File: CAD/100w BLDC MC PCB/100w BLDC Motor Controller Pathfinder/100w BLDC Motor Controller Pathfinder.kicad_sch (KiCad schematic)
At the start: 30 parts, among them SW1 PTS815 SJM 250 SMTR LFS, SW2 PTS815 SJM 250 SMTR LFS, U1 RP2040, U2 W25Q128JVS, Y1 ABLS-12.000MHZ-B4-T

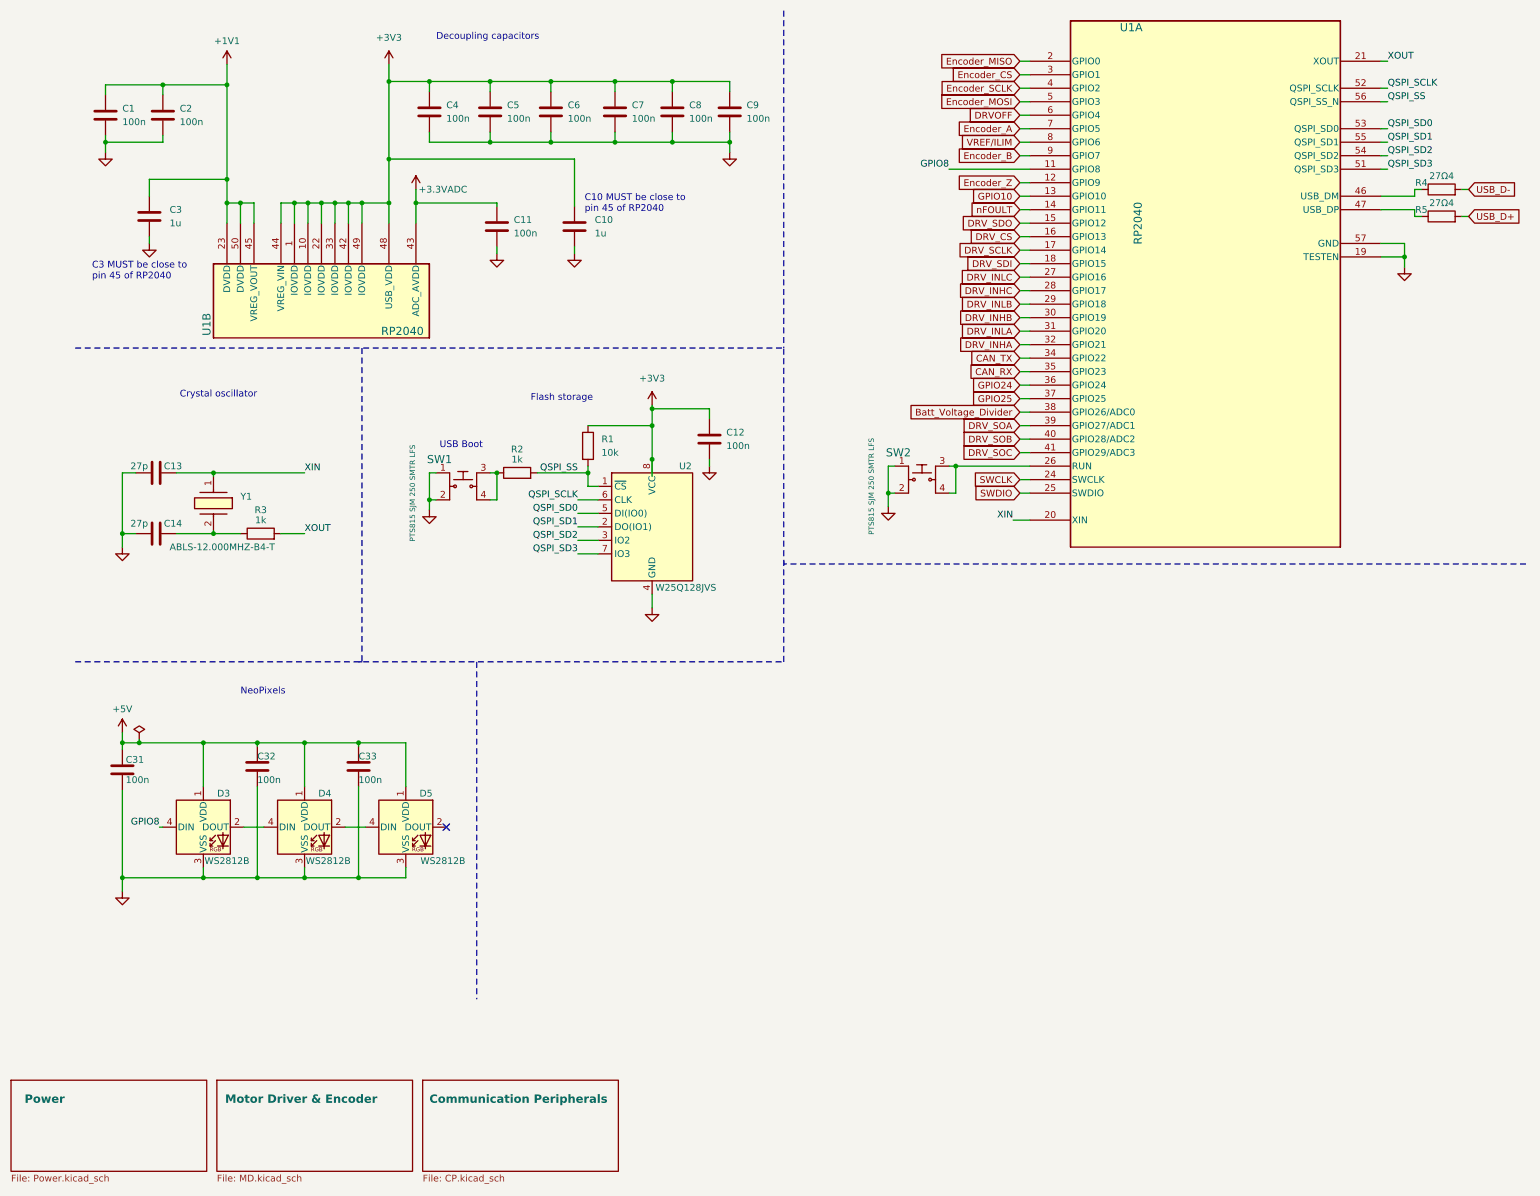
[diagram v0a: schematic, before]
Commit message: Rev: 0.1
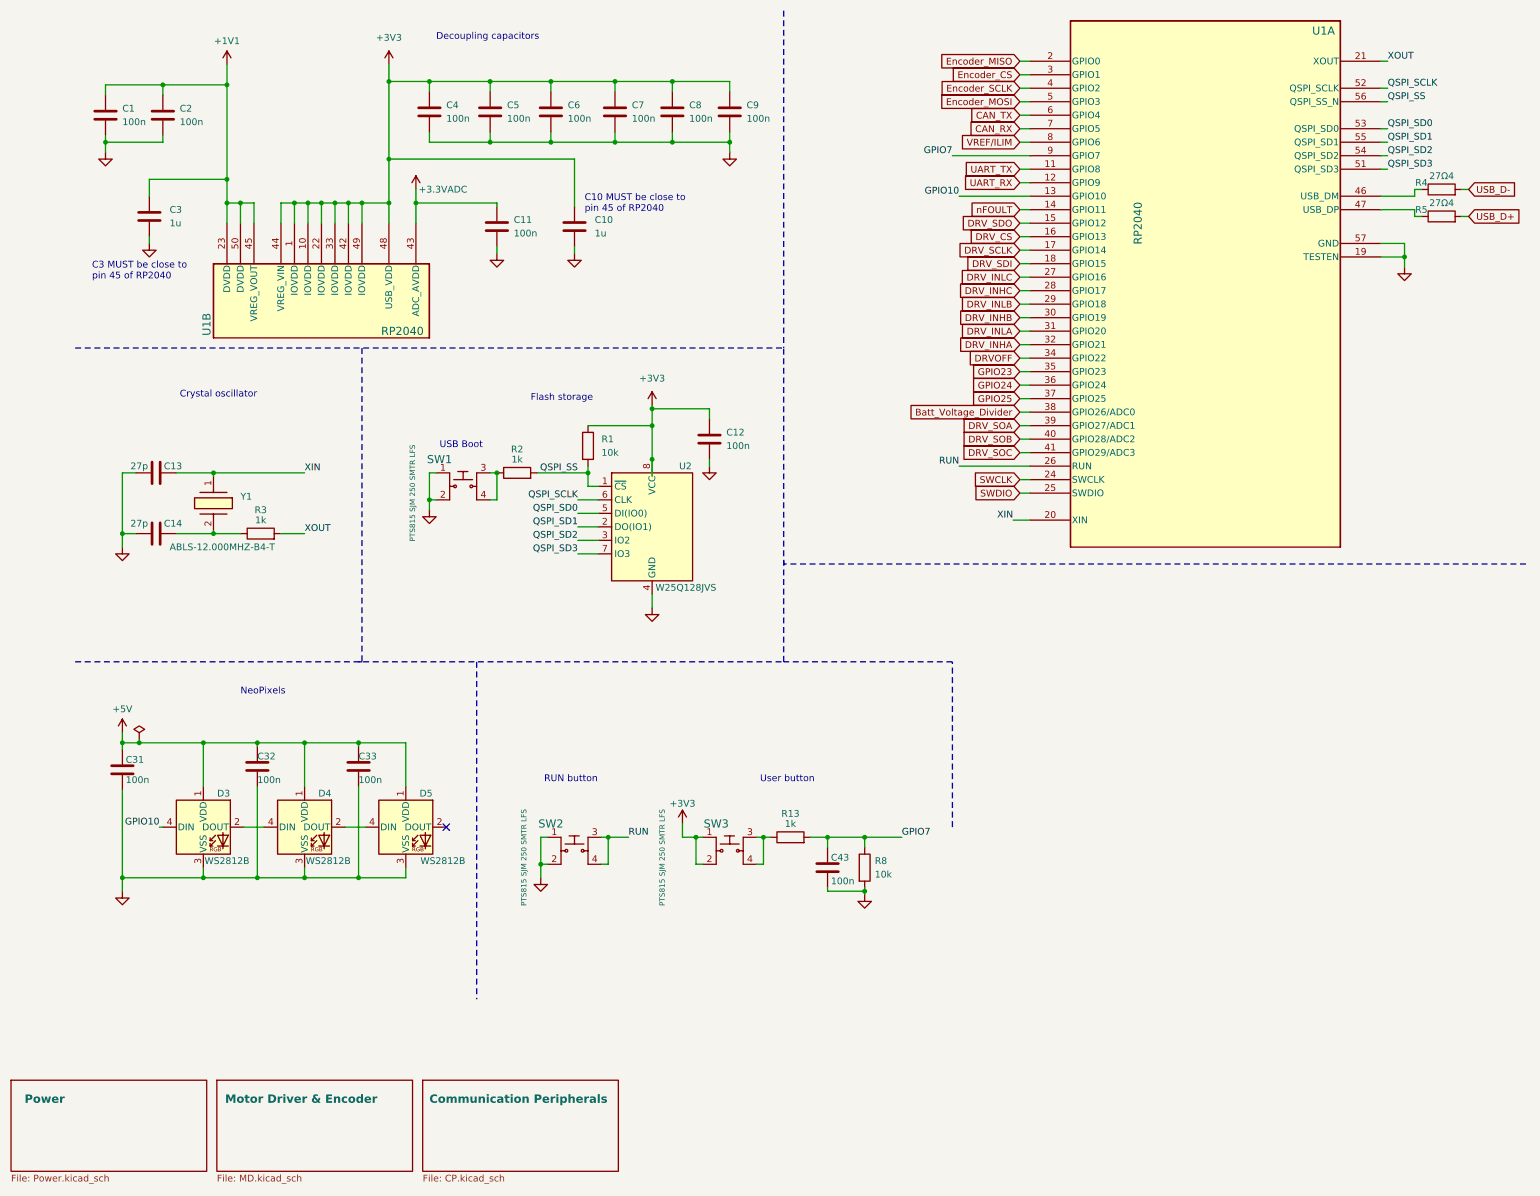
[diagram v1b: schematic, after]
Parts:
- added C43: 100n, symbol Device:C
- added R13: 1k, symbol Device:R
- added R8: 10k, symbol Device:R
- added SW3: PTS815 SJM 250 SMTR LFS, SW4_PTS815 SJM 250 SMTR LFS_CNK, symbol 2024-01-22_02-04-17:PTS815_SJM_250_SMTR_LFS
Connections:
- net Encoder_A is gone; now on net CAN_RX: U1.7 (GPIO5)
- net +3V3: now also SW3.1, SW3.2
- net CAN_RX: no longer U1.35 (GPIO23)
- net CAN_TX: now also U1.6 (GPIO4); no longer U1.34 (GPIO22)
- net DRVOFF: now also U1.34 (GPIO22); no longer U1.6 (GPIO4)
- net GND: now also C43.2, R8.2
- net GPIO10: now also D3.4 (DIN)
- net RUN: now reaches SW2.3, SW2.4, U1.26 (RUN)
- net Encoder_B renamed GPIO7
- net GPIO7: now also C43.1, R13.2, R8.1
- net Encoder_Z renamed UART_RX
- net GPIO8 renamed UART_TX
- net UART_TX: no longer D3.4 (DIN)
- new net: R13.1, SW3.3, SW3.4
- new net GPIO23: U1.35 (GPIO23)
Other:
- note added: "RUN button"
- note added: "User button"
- company: (none) -> SCS
- title: (none) -> 100w BLDC Motor Controller Pathfinder
- moved on the sheet: SW2
